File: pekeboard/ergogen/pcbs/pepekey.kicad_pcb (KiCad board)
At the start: 2 copper layers, 156.8 x 132.1 mm, 63 parts

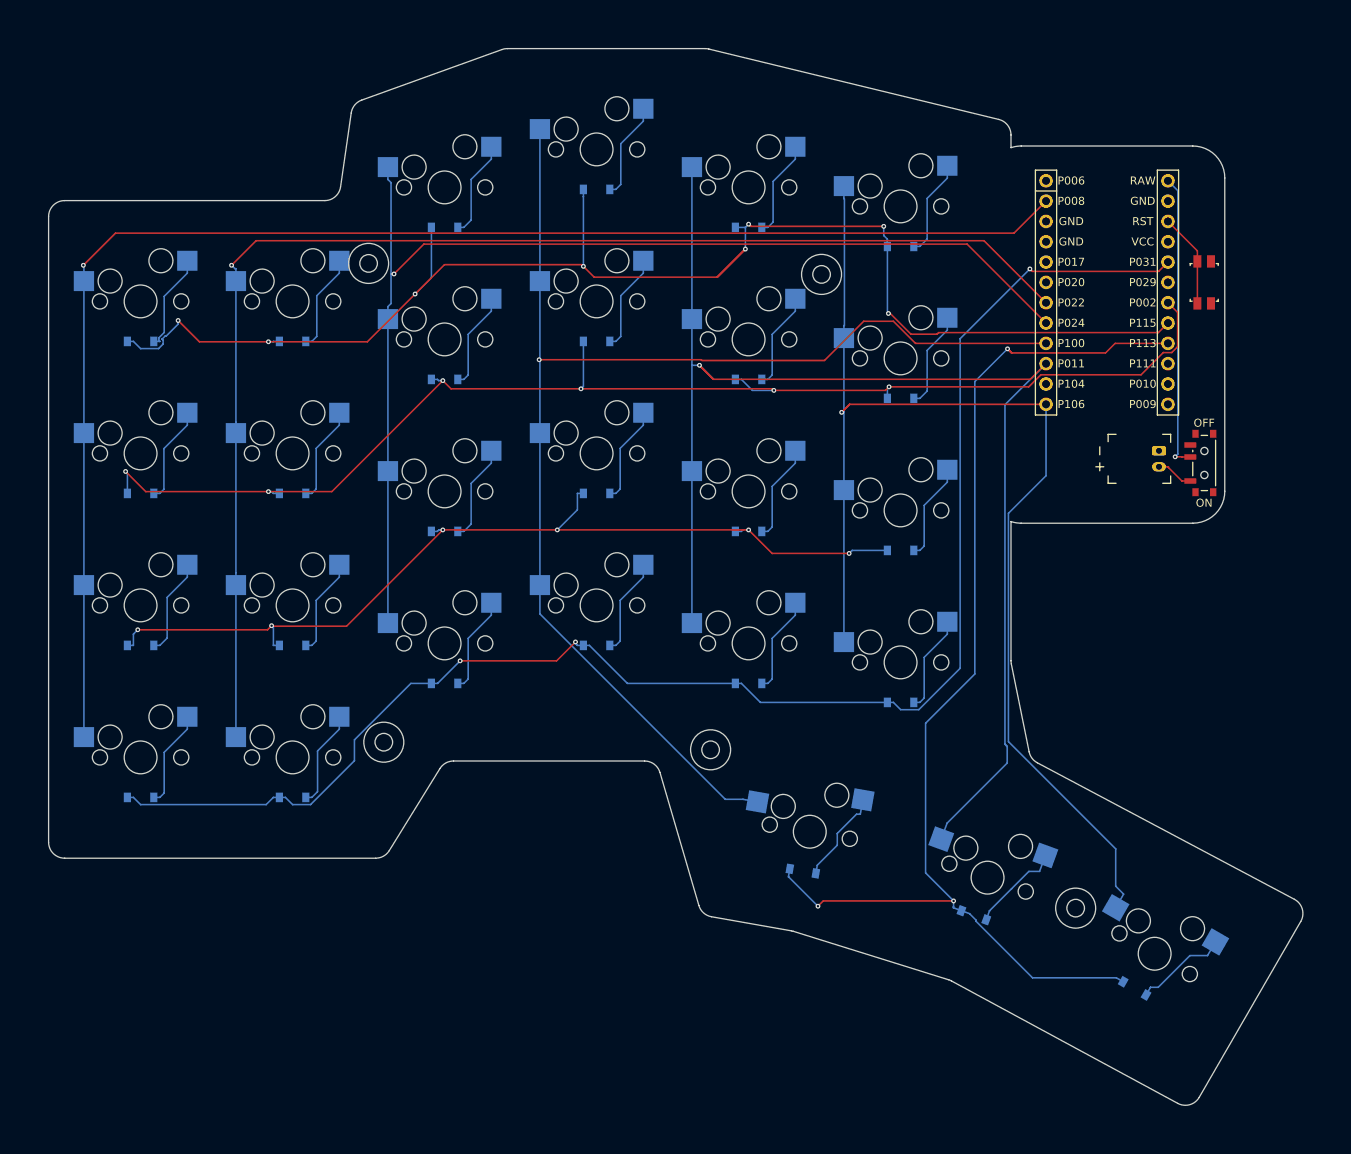
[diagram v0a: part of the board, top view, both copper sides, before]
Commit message: Extreme trimming
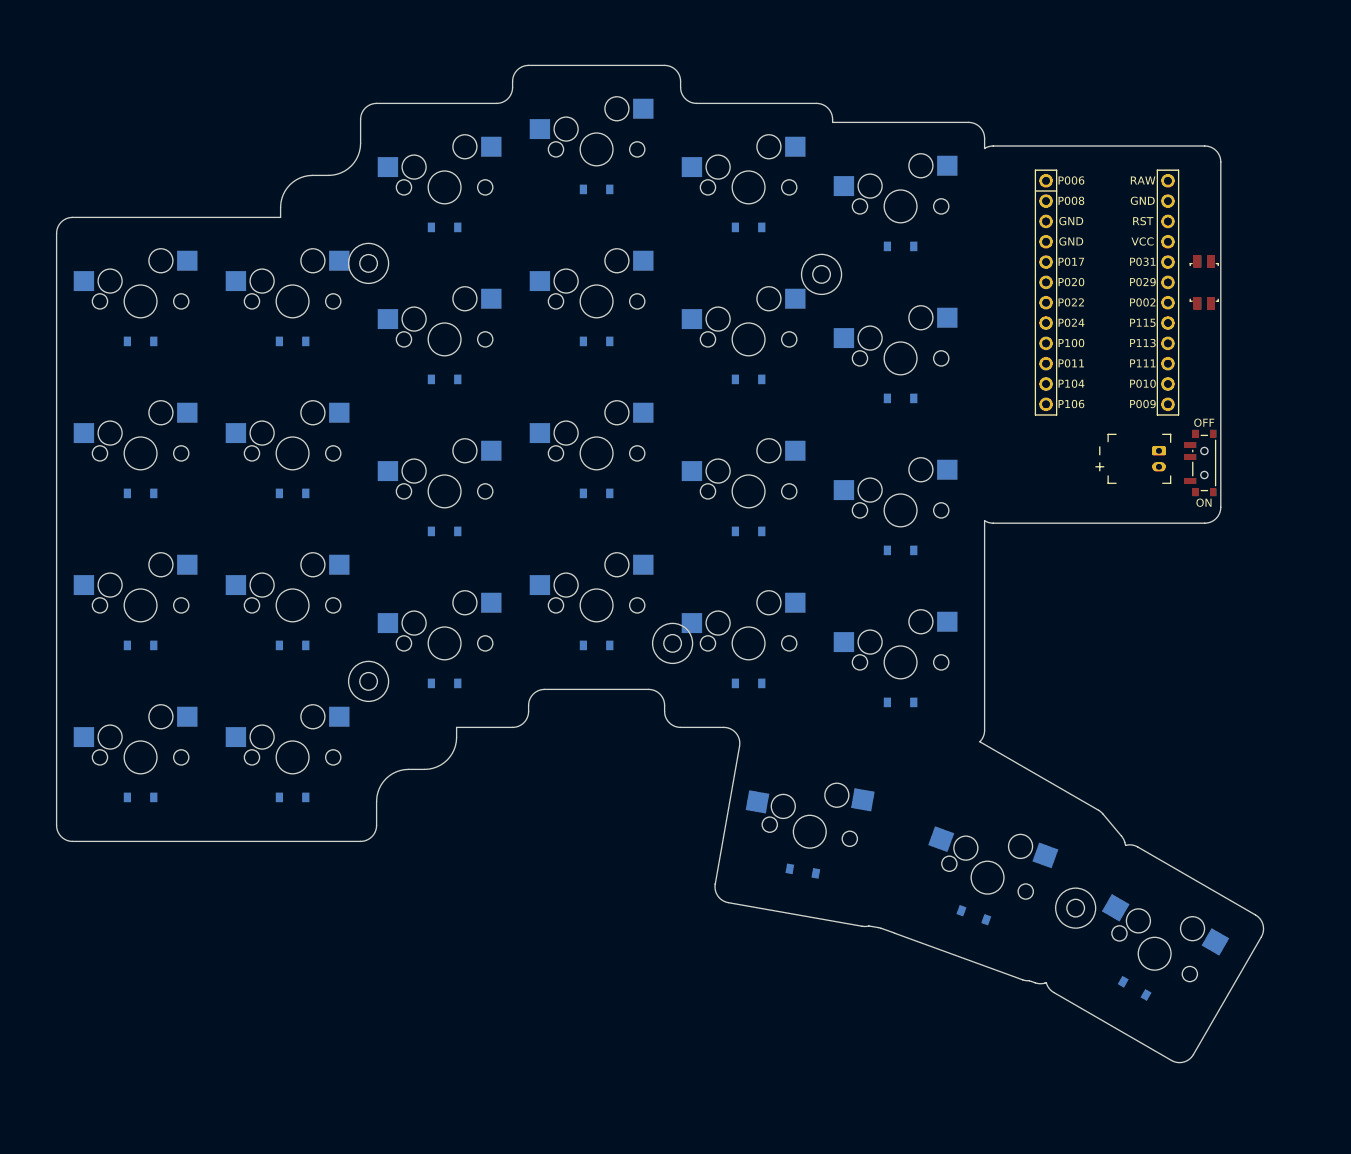
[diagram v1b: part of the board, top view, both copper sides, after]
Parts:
- moved MH4 14.1 mm to (166.5, 105.8)
- moved MH2 7.83 mm to (128.5, 110.5)
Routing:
- net P115: track 197.9 -> 0.00 mm, vias 8 -> 0
- net P031: track 192.3 -> 0.00 mm, vias 3 -> 0
- net P008: track 182.7 -> 0.00 mm, vias 1 -> 0
- net P011: track 177.8 -> 0.00 mm, vias 1 -> 0
- net P022: track 166.9 -> 0.00 mm, vias 1 -> 0
- net P002: track 165.8 -> 0.00 mm, vias 6 -> 0
- net P100: track 164.1 -> 0.00 mm, vias 1 -> 0
- net P106: track 160.1 -> 0.00 mm, vias 1 -> 0
- net P113: track 147.6 -> 0.00 mm, vias 3 -> 0
- net P024: track 144.8 -> 0.00 mm, vias 1 -> 0
- net P025: track 116.1 -> 0.00 mm, vias 6 -> 0
- net RAW: track 37.1 -> 0.00 mm, vias 1 -> 0
- net outer_num: track 12.4 -> 0.00 mm
- net middle_num: track 12.3 -> 0.00 mm
- net inner_home: track 12.3 -> 0.00 mm
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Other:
- board size 156.8 x 132.1 mm -> 150.9 x 124.7 mm
